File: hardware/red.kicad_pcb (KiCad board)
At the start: 6 copper layers, 40 x 40 mm, 193 parts, among them J1 MICROSDCARD, J2 USB-A, J3 MICRO_HDMI, J4 USB-MINI-B-SMD, J5 STACK-UP-LOW, J6 STACK-DOWN, J7 STACK-UP-LOW, J8 STACK-DOWN, P1 Camera/EXT, Q1 2N7002, Q2 2N7002, Q3 2N7002, SW1 Power, U1 H5TQ4G63AFR, U2 AXP152, U3 RT9701XB, U4 82400152, U5 TPD4S010DQA, U6 TPD4S010DQA, U7 TPD4S010DQA, U8 82400152, U9 NX3008PBKS, X1 24MHz

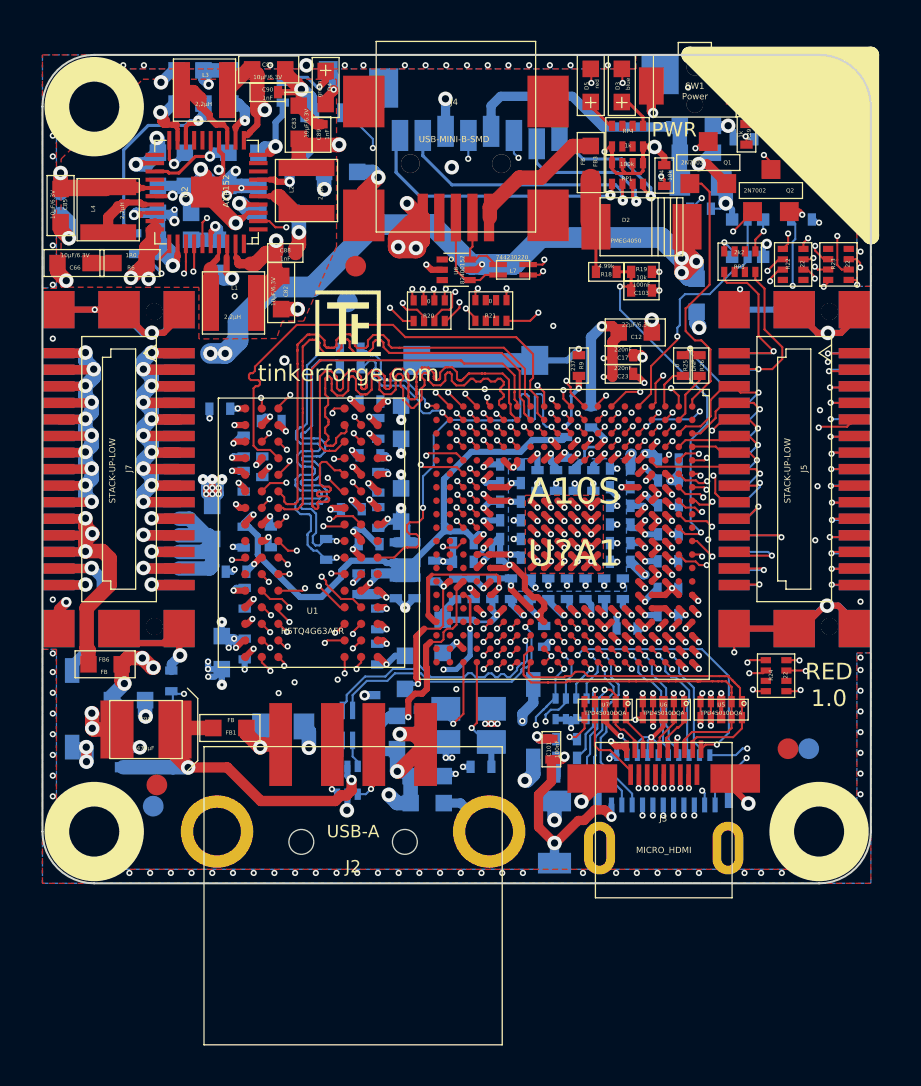
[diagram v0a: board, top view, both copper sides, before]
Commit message: Add 3d information (tbc)
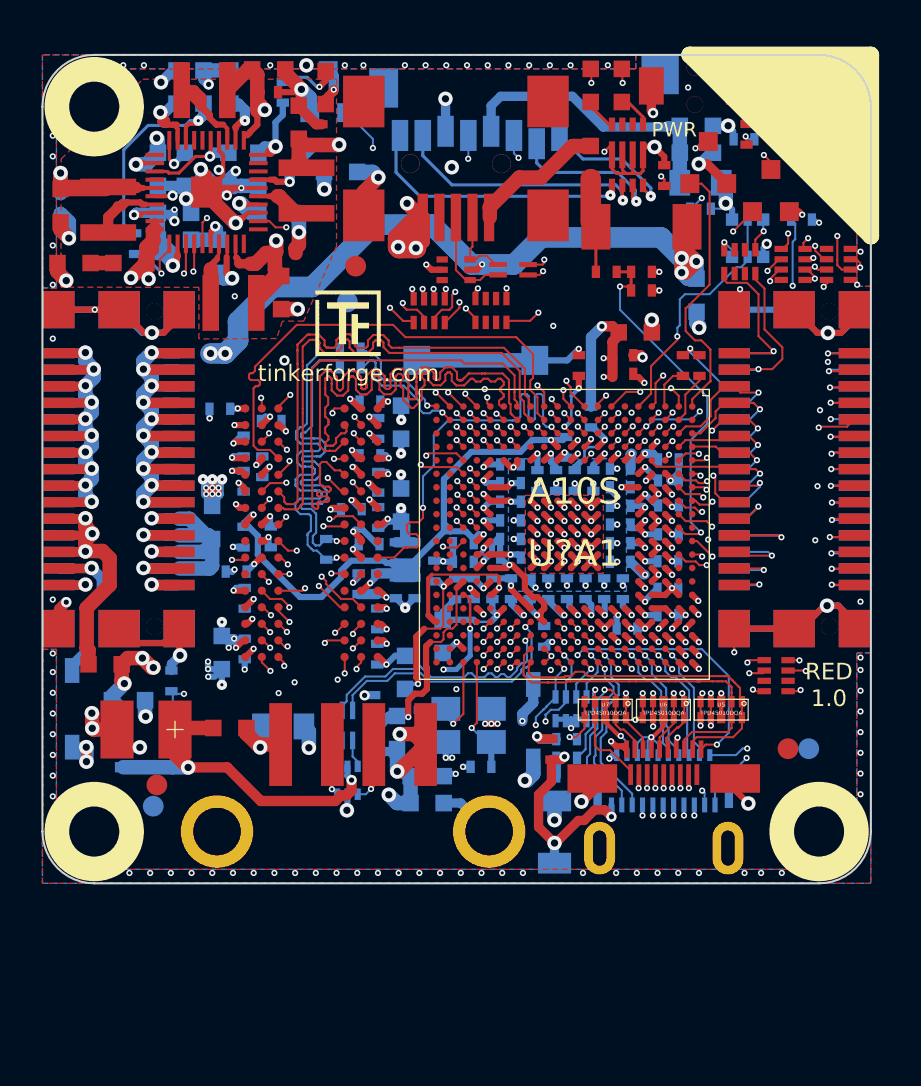
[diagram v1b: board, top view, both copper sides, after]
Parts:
- C1, C10, C101, C103, C11, C13, C15, C16, C17, C18, C19, C2, C20, C21, C22, C23, C24, C27, C28, C29, C3, C30, C31, C32, C34, C35, C36, C37, C38, C39, C4, C40, C41, C42, C43, C44, C45, C46, C47, C49, C5, C50, C51, C52, C53, C54, C55, C57, C59, C6, C65, C67, C68, C69, C7, C70, C71, C72, C73, C79, C8, C80, C81, C86, C87, C88, C89, C9, C90, C91, C93, C94, C95: footprint tinkerforge:0402 -> C0402
- C100, L5: footprint tinkerforge:0805 -> C0805
- C102, C12, C14, C25, C26, C33, C56, C58, C60, C61, C62, C63, C64, C66, C74, C75, C76, C77, C78, C82, C83, C84, C85, C92, C96, C97, C98, FB1, FB2, FB3, FB4, FB5, FB6: footprint tinkerforge:0603 -> C0603
- C48, R6: footprint tinkerforge:0603 -> R0603
- C99: footprint tinkerforge:3528-21 -> 3528-21
- D1, D6: footprint tinkerforge:SOD-123 -> SOD-123
- D2: footprint tinkerforge:SOD-128 -> SOD-128
- D3, D4, D5: footprint tinkerforge:D0603 -> D0603
- F1: footprint tinkerforge:1206 -> C1206
- J1: footprint tinkerforge:MicroSD_TF001A -> kicad-libraries:MicroSD_TF001A
- J2: footprint kicad-libraries:USB-A-SMT-8231-PEG -> USB-A-SMT-8231
- J3: footprint tinkerforge:MICRO-HDMI-D -> kicad-libraries:MICRO-HDMI-D
- J4: footprint tinkerforge:USB-MINI-B-SMD -> USB-MINI-B-SMD
- J5, J7: footprint tinkerforge:BTB08-ACS-TOP -> BTB08-ACS-TOP
- J6, J8: footprint tinkerforge:BTB08-ACS-BTM -> BTB08-ACS-BTM
- L1, L2, L3, L4: footprint tinkerforge:NRH3015 -> kicad-libraries:NRH3015
- L6, L7: footprint tinkerforge:WE-CNSW-0603 -> WE-CNSW-0603
- P1: footprint tinkerforge:502078-2110-C -> 502078-2110-C
- Q1, Q2, Q3: footprint tinkerforge:SOT23GDS -> SOT23GDS
- R1, R10, R11, R12, R13, R14, R15, R16, R17, R18, R19, R2, R25, R26, R27, R28, R29, R3, R4, R5, R7, R8, R9: footprint tinkerforge:0402 -> R0402
- R20, R21, R22, R23, R24, RP1, RP2, RP3, RP4: footprint tinkerforge:741X083 -> 4X0402
- SW1: footprint tinkerforge:TACT-SWITCH -> TACT-SWITCH
- U1: footprint tinkerforge:FBGA96 -> FBGA96
- U2: footprint tinkerforge:QFN40_5X5 -> QFN40_5X5
- U3: footprint tinkerforge:SOT23-5 -> SOT23-5
- U4, U8: footprint tinkerforge:SOT563 -> SOT563
- U5, U6, U7: footprint tinkerforge:TPD4S010DQA -> TPD4S010DQA
- U9: footprint tinkerforge:SOT363 -> kicad-libraries:SOT363
- U?A1: footprint tinkerforge:TFBGA336 -> TFBGA336
- X1: footprint tinkerforge:CRYSTAL_3225 -> CRYSTAL_3225
- ~1, ~2, ~3, ~4: footprint kicad-libraries:DRILL_NP -> DRILL_NP
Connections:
- C13 pad 1: +3.3V -> 3V3
- C18 pad 1: +3.3V -> 3V3
- C2 pad 1: +3.3V -> 3V3
- C20 pad 1: +3.3V -> 3V3
- C24 pad 1: +3.3V -> 3V3
- C5 pad 1: +3.3V -> 3V3
- C61 pad 2: +3.3V -> 3V3
- C7 pad 1: +3.3V -> 3V3
- C82 pad 2: +3.3V -> 3V3
- C88 pad 2: +3.3V -> 3V3
- C9 pad 1: +3.3V -> 3V3
- D1 pad 1: +3.3V -> 3V3
- D6 pad 1: +3.3V -> +3V3
- J3 pad 2: (no net) -> Net-(J3-Pad2)
- J4 pad 4: (no net) -> Net-(J4-Pad4)
- L1 pad 2: +3.3V -> 3V3
- L5 pad 1: +3.3V -> 3V3
- P1 pad 2: +3.3V -> 3V3
- R14 pad 1: +3.3V -> 3V3
- R21 pad 2: (no net) -> Net-(R21-Pad2)
- R21 pad 3: (no net) -> Net-(R21-Pad3)
- R21 pad 6: (no net) -> Net-(R21-Pad6)
- R21 pad 7: (no net) -> Net-(R21-Pad7)
- R22 pad 4: (no net) -> Net-(R22-Pad4)
- R22 pad 5: (no net) -> Net-(R22-Pad5)
- R23 pad 1: (no net) -> Net-(R23-Pad1)
- R23 pad 8: (no net) -> Net-(R23-Pad8)
- R24 pad 3: (no net) -> Net-(R24-Pad3)
- R24 pad 6: (no net) -> Net-(R24-Pad6)
- R27 pad 1: +3.3V -> 3V3
- R3 pad 1: +3.3V -> 3V3
- R4 pad 2: +3.3V -> 3V3
- RP1 pad 5: +3.3V -> 3V3
- RP1 pad 6: +3.3V -> 3V3
- RP1 pad 7: +3.3V -> 3V3
- RP1 pad 8: +3.3V -> 3V3
- RP2 pad 5: +3.3V -> 3V3
- RP2 pad 6: +3.3V -> 3V3
- RP2 pad 7: +3.3V -> 3V3
- RP2 pad 8: +3.3V -> 3V3
- RP3 pad 2: (no net) -> Net-(RP3-Pad2)
- RP3 pad 3: (no net) -> Net-(RP3-Pad3)
- RP3 pad 6: (no net) -> Net-(RP3-Pad6)
- RP3 pad 7: (no net) -> Net-(RP3-Pad7)
- RP4 pad 2: (no net) -> Net-(RP4-Pad2)
- RP4 pad 3: (no net) -> Net-(RP4-Pad3)
- RP4 pad 5: +3.3V -> 3V3
- RP4 pad 6: (no net) -> Net-(RP4-Pad6)
- RP4 pad 7: (no net) -> Net-(RP4-Pad7)
- RP4 pad 8: +3.3V -> 3V3
- U1 pad J1: (no net) -> Net-(U1-PadJ1)
- U1 pad J9: (no net) -> Net-(U1-PadJ9)
- U1 pad L1: (no net) -> Net-(U1-PadL1)
- U1 pad L9: (no net) -> Net-(U1-PadL9)
- U1 pad M7: (no net) -> Net-(U1-PadM7)
- U2 pad 1: (no net) -> Net-(U2-Pad1)
- U2 pad 10: +3.3V -> 3V3
- U2 pad 16: (no net) -> Net-(U2-Pad16)
- U2 pad 17: (no net) -> Net-(U2-Pad17)
- U2 pad 21: (no net) -> Net-(U2-Pad21)
- U2 pad 24: (no net) -> Net-(U2-Pad24)
- U2 pad 39: +3.3V -> 3V3
- U2 pad 40: (no net) -> Net-(U2-Pad40)
- U2 pad 8: (no net) -> Net-(U2-Pad8)
- U2 pad 9: (no net) -> Net-(U2-Pad9)
- U8 pad 1: (no net) -> Net-(U8-Pad1)
- U8 pad 3: (no net) -> Net-(U8-Pad3)
- U9 pad 1: +3.3V -> 3V3
- U9 pad 4: +3.3V -> 3V3
- U?A1 pad A10: (no net) -> Net-(U?A1-PadA10)
- U?A1 pad A13: (no net) -> Net-(U?A1-PadA13)
- U?A1 pad A14: (no net) -> Net-(U?A1-PadA14)
- U?A1 pad A2: (no net) -> Net-(U?A1-PadA2)
- U?A1 pad A9: (no net) -> Net-(U?A1-PadA9)
- U?A1 pad B11: (no net) -> Net-(U?A1-PadB11)
- U?A1 pad B13: (no net) -> Net-(U?A1-PadB13)
- U?A1 pad B14: (no net) -> Net-(U?A1-PadB14)
- U?A1 pad E2: (no net) -> Net-(U?A1-PadE2)
- U?A1 pad E5: +3.3V -> 3V3
- U?A1 pad F1: (no net) -> Net-(U?A1-PadF1)
- U?A1 pad F2: (no net) -> Net-(U?A1-PadF2)
- U?A1 pad F5: +3.3V -> 3V3
- U?A1 pad G16: +3.3V -> 3V3
- U?A1 pad H16: +3.3V -> 3V3
- U?A1 pad J16: +3.3V -> 3V3
- U?A1 pad K16: +3.3V -> 3V3
- U?A1 pad K19: (no net) -> Net-(U?A1-PadK19)
- U?A1 pad K20: (no net) -> Net-(U?A1-PadK20)
- U?A1 pad L16: +3.3V -> 3V3
- U?A1 pad M18: (no net) -> Net-(U?A1-PadM18)
- U?A1 pad M19: +3.3V -> 3V3
- U?A1 pad M20: +3.3V -> 3V3
- U?A1 pad M4: (no net) -> Net-(U?A1-PadM4)
- U?A1 pad N4: (no net) -> Net-(U?A1-PadN4)
- U?A1 pad T14: +3.3V -> 3V3
- U?A1 pad T16: (no net) -> Net-(U?A1-PadT16)
- U?A1 pad U14: (no net) -> Net-(U?A1-PadU14)
- U?A1 pad U17: (no net) -> Net-(U?A1-PadU17)
- U?A1 pad U18: (no net) -> Net-(U?A1-PadU18)
- U?A1 pad U19: (no net) -> Net-(U?A1-PadU19)
- U?A1 pad U5: (no net) -> Net-(U?A1-PadU5)
- U?A1 pad V12: (no net) -> Net-(U?A1-PadV12)
- U?A1 pad V13: (no net) -> Net-(U?A1-PadV13)
- U?A1 pad V16: (no net) -> Net-(U?A1-PadV16)
- U?A1 pad V17: (no net) -> Net-(U?A1-PadV17)
- U?A1 pad V18: (no net) -> Net-(U?A1-PadV18)
- U?A1 pad W10: (no net) -> Net-(U?A1-PadW10)
- U?A1 pad W11: (no net) -> Net-(U?A1-PadW11)
- U?A1 pad W12: (no net) -> Net-(U?A1-PadW12)
- U?A1 pad W13: (no net) -> Net-(U?A1-PadW13)
- U?A1 pad W15: (no net) -> Net-(U?A1-PadW15)
- U?A1 pad W16: (no net) -> Net-(U?A1-PadW16)
- U?A1 pad W17: (no net) -> Net-(U?A1-PadW17)
- U?A1 pad W18: (no net) -> Net-(U?A1-PadW18)
- U?A1 pad W19: (no net) -> Net-(U?A1-PadW19)
- U?A1 pad W20: (no net) -> Net-(U?A1-PadW20)
- U?A1 pad W3: (no net) -> Net-(U?A1-PadW3)
- U?A1 pad W4: (no net) -> Net-(U?A1-PadW4)
- U?A1 pad W5: (no net) -> Net-(U?A1-PadW5)
- U?A1 pad W6: (no net) -> Net-(U?A1-PadW6)
- U?A1 pad W7: (no net) -> Net-(U?A1-PadW7)
- U?A1 pad W8: (no net) -> Net-(U?A1-PadW8)
- U?A1 pad W9: (no net) -> Net-(U?A1-PadW9)
- U?A1 pad Y10: (no net) -> Net-(U?A1-PadY10)
- U?A1 pad Y11: (no net) -> Net-(U?A1-PadY11)
- U?A1 pad Y12: (no net) -> Net-(U?A1-PadY12)
- U?A1 pad Y13: (no net) -> Net-(U?A1-PadY13)
- U?A1 pad Y14: (no net) -> Net-(U?A1-PadY14)
- U?A1 pad Y15: (no net) -> Net-(U?A1-PadY15)
- U?A1 pad Y16: (no net) -> Net-(U?A1-PadY16)
- U?A1 pad Y18: (no net) -> Net-(U?A1-PadY18)
- U?A1 pad Y19: (no net) -> Net-(U?A1-PadY19)
- U?A1 pad Y2: (no net) -> Net-(U?A1-PadY2)
- U?A1 pad Y20: (no net) -> Net-(U?A1-PadY20)
- U?A1 pad Y3: (no net) -> Net-(U?A1-PadY3)
- U?A1 pad Y4: (no net) -> Net-(U?A1-PadY4)
- U?A1 pad Y5: (no net) -> Net-(U?A1-PadY5)
- U?A1 pad Y6: (no net) -> Net-(U?A1-PadY6)
- U?A1 pad Y7: (no net) -> Net-(U?A1-PadY7)
- U?A1 pad Y8: (no net) -> Net-(U?A1-PadY8)
- U?A1 pad Y9: (no net) -> Net-(U?A1-PadY9)
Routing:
- net +3.3V: track 191.6 -> 0.00 mm, vias 21 -> 0
- net 3V3: track 0.00 -> 190.9 mm, vias 0 -> 21
- net +3V3: track 0.00 -> 0.68 mm
